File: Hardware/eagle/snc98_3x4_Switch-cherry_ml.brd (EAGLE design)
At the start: 56.4 x 83.2 mm, 73 parts

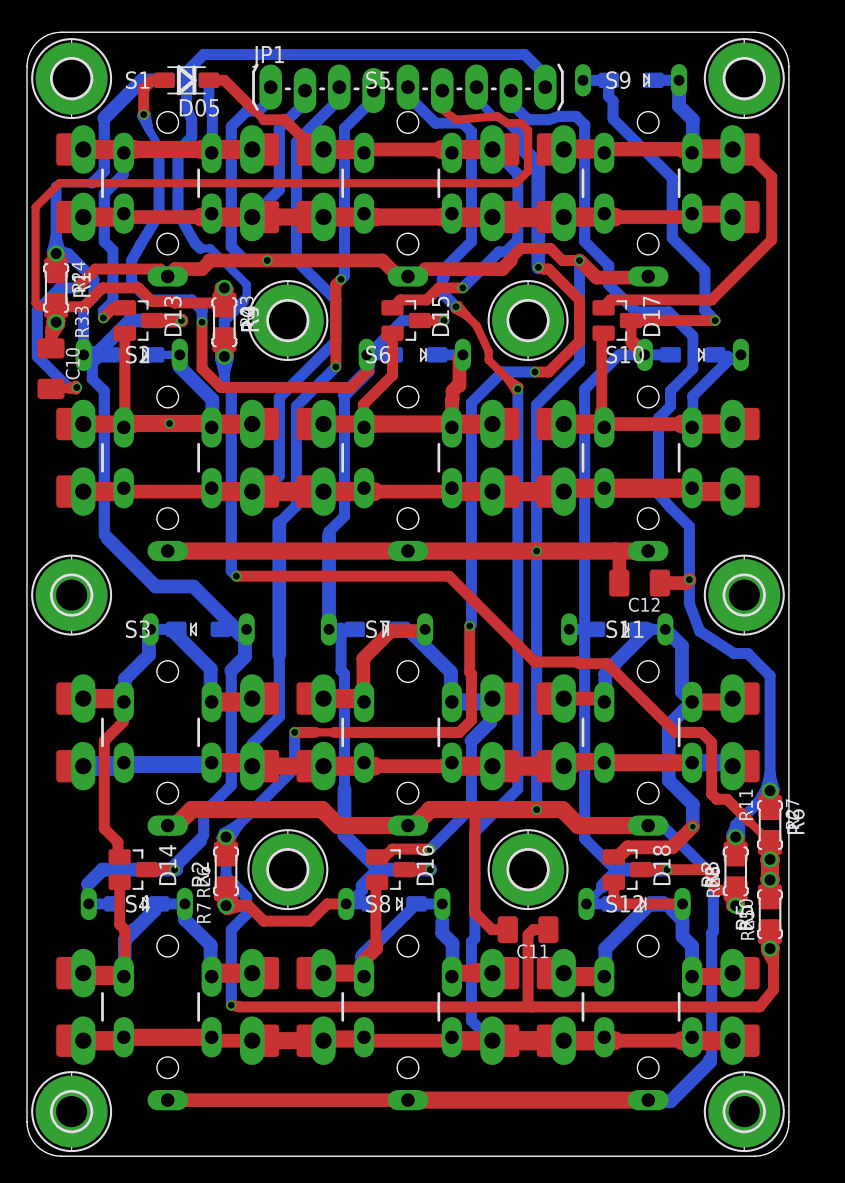
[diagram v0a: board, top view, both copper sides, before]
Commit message: add_prozent
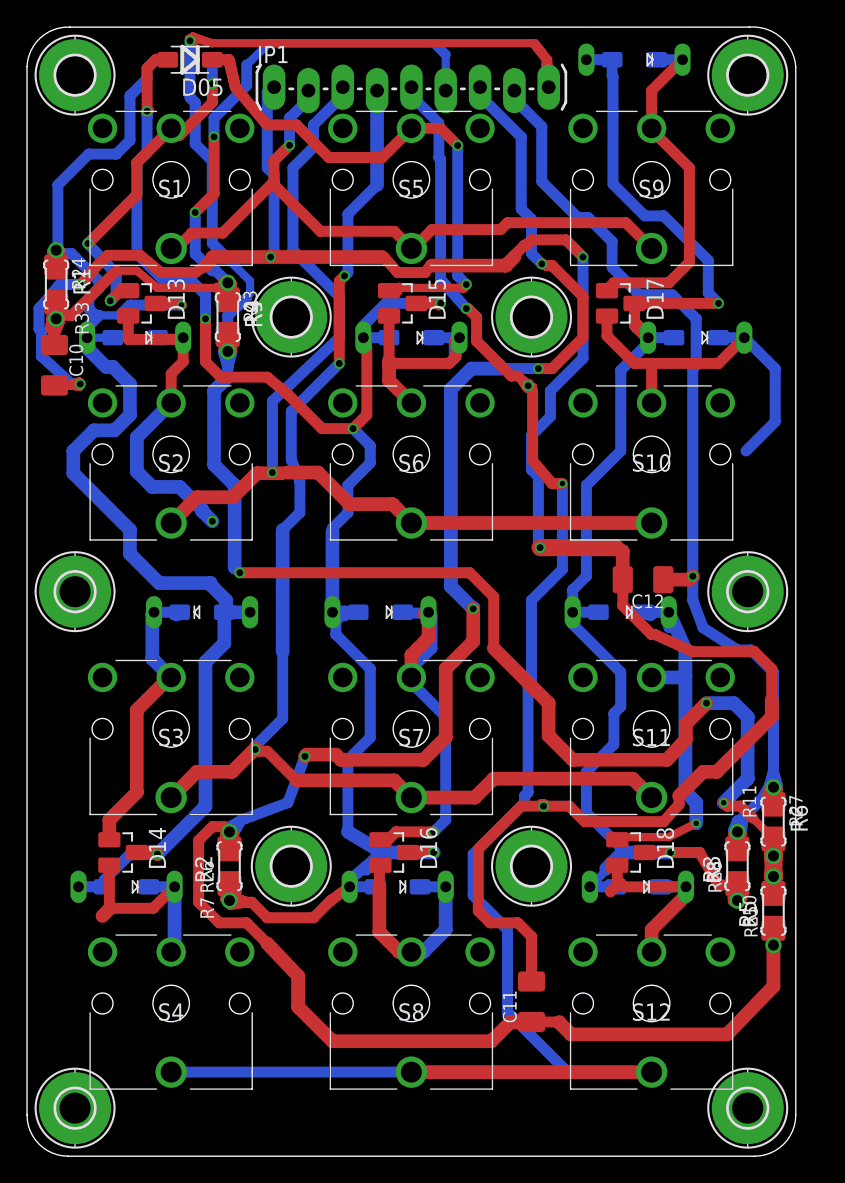
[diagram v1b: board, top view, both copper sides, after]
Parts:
- S1, S10, S11, S12, S2, S3, S4, S5, S6, S7, S8, S9: value B3F-4150 -> ML1A-11JW; device SmartPrj:TACTILE-PTH-12MM -> ML1A-11JW:ML1A11JW
- moved S6 6.31 mm to (23.4, 55.8)
- moved S7 6.31 mm to (23.4, 35.4)
- moved S8 6.31 mm to (23.4, 15.1)
- moved S2 6.31 mm to (5.59, 55.8)
- moved S3 6.31 mm to (5.59, 35.4)
- moved S4 6.31 mm to (5.59, 15.1)
- moved S1 6.31 mm to (5.59, 76.1)
- moved S5 6.31 mm to (23.4, 76.1)
- moved S10 6.31 mm to (41.1, 55.8)
- moved S11 6.31 mm to (41.1, 35.4)
- moved S12 6.31 mm to (41.1, 15.1)
- moved S9 6.31 mm to (41.1, 76.1)
- moved C11 5.34 mm to (37.3, 11.4), turned to 90 degrees
- moved D01 1.55 mm to (12.1, 81.2)
- moved D05 1.55 mm to (12.1, 81.2)
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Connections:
- removed net N$24: D05.C, D15.1, S5.P$13, S5.P$14, S5.P$23, S5.P$24, S5.P$3, S5.P$4
- new net N$7: D05.C, D15.1, S5.2
- net C1: now also S1.4, S5.4, S9.4; no longer S1.P$1, S1.P$11, S1.P$12, S1.P$2, S1.P$21, S1.P$22, S5.P$1, S5.P$11, S5.P$12, S5.P$2, S5.P$21, S5.P$22, S9.P$1, S9.P$11, S9.P$12, S9.P$2, S9.P$21, S9.P$22
- net C2: now also S10.4, S2.4, S6.4; no longer S10.P$1, S10.P$11, S10.P$12, S10.P$2, S10.P$21, S10.P$22, S2.P$1, S2.P$11, S2.P$12, S2.P$2, S2.P$21, S2.P$22, S6.P$1, S6.P$11, S6.P$12, S6.P$2, S6.P$21, S6.P$22
- net C3: now also S11.4, S3.4, S7.4; no longer S11.P$1, S11.P$11, S11.P$12, S11.P$2, S11.P$21, S11.P$22, S3.P$1, S3.P$11, S3.P$12, S3.P$2, S3.P$21, S3.P$22, S7.P$1, S7.P$11, S7.P$12, S7.P$2, S7.P$21, S7.P$22
- net C4: now also S12.4, S4.4, S8.4; no longer S12.P$1, S12.P$11, S12.P$12, S12.P$2, S12.P$21, S12.P$22, S4.P$1, S4.P$11, S4.P$12, S4.P$2, S4.P$21, S4.P$22, S8.P$1, S8.P$11, S8.P$12, S8.P$2, S8.P$21, S8.P$22
- net GND: no longer S1.P$15, S10.P$15, S11.P$15, S12.P$15, S2.P$15, S3.P$15, S4.P$15, S5.P$15, S6.P$15, S7.P$15, S8.P$15, S9.P$15
- net N$16: now also S9.2; no longer S9.P$13, S9.P$14, S9.P$23, S9.P$24, S9.P$3, S9.P$4
- net N$18: now also S10.2; no longer S10.P$13, S10.P$14, S10.P$23, S10.P$24, S10.P$3, S10.P$4
- net N$19: now also S2.2; no longer S2.P$13, S2.P$14, S2.P$23, S2.P$24, S2.P$3, S2.P$4
- net N$2: now also S4.2; no longer S4.P$13, S4.P$14, S4.P$23, S4.P$24, S4.P$3, S4.P$4
- net N$21: now also S11.2; no longer S11.P$13, S11.P$14, S11.P$23, S11.P$24, S11.P$3, S11.P$4
- net N$22: now also S12.2; no longer S12.P$13, S12.P$14, S12.P$23, S12.P$24, S12.P$3, S12.P$4
- net N$25: now also S6.2; no longer S6.P$13, S6.P$14, S6.P$23, S6.P$24, S6.P$3, S6.P$4
- net N$28: now also S7.2; no longer S7.P$13, S7.P$14, S7.P$23, S7.P$24, S7.P$3, S7.P$4
- net N$30: now also S8.2; no longer S8.P$13, S8.P$14, S8.P$23, S8.P$24, S8.P$3, S8.P$4
- net N$32: now also S3.2; no longer S3.P$13, S3.P$14, S3.P$23, S3.P$24, S3.P$3, S3.P$4
- net N$6: now also S1.2; no longer S1.P$13, S1.P$14, S1.P$23, S1.P$24, S1.P$3, S1.P$4
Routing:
- net GND: track 272.0 -> 163.4 mm
- net N$24: track 44.4 -> 0.00 mm, vias 1 -> 0
- net N$7: track 0.00 -> 42.0 mm, vias 0 -> 2
- net C4: track 162.6 -> 129.9 mm, vias 2 -> 3
- net C3: track 123.7 -> 93.2 mm, vias 2 -> 3
- net N$16: track 54.9 -> 26.0 mm
- net C1: track 67.9 -> 49.2 mm, vias 0 -> 1
- net A1: track 94.4 -> 75.8 mm, vias 0 -> 2
- net N$25: track 35.1 -> 17.5 mm
- net AREF: track 173.0 -> 189.0 mm, vias 1 -> 4
- net N$2: track 33.1 -> 17.2 mm
- net C2: track 89.1 -> 73.7 mm, vias 0 -> 1
- net N$28: track 45.7 -> 31.4 mm
- net N$30: track 32.0 -> 17.9 mm
- net N$32: track 35.9 -> 21.9 mm
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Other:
- board size 56.4 x 83.2 mm -> 56.9 x 83.6 mm
